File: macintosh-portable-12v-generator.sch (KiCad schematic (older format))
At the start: 14 parts, among them Q3 P2A

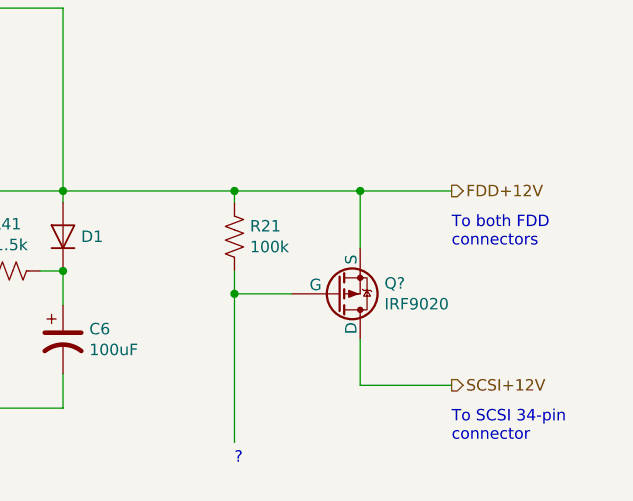
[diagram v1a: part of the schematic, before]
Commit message: Finished V1M, more references on other sheets.
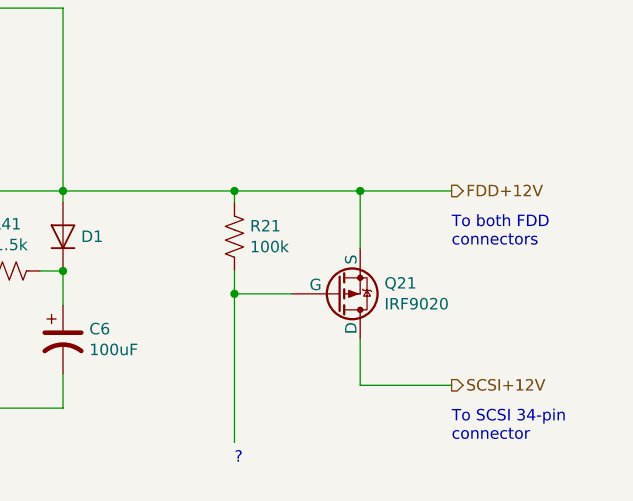
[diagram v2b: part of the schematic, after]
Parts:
- gave numbers to parts that had none: 1
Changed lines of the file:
@@
 Sheet 3 4
 Title "Macintosh Portable 12V Generator Circuit"
-Date "2019-05-22"
-Rev "0.1"
+Date "2019-05-27"
+Rev "0.12"
 Comp "https://oldcrap.org"
-Comment1 ""
+Comment1 "Author: Pawel Pieczul"
 Comment2 ""
 Comment3 ""
@@
 Connection ~ 6400 4350
 $Comp
-L Transistor_FET:IRF9020 Q?
+L Transistor_FET:IRF9020 Q21
 U 1 1 5CFB719D
 P 7600 4450
-F 0 "Q?" H 7806 4404 50  0000 L CNN
+F 0 "Q21" H 7806 4404 50  0000 L CNN
 F 1 "IRF9020" H 7806 4495 50  0000 L CNN
 F 2 "Package_TO_SOT_SMD:TO-252-3_TabPin2" H 7800 4375 50  0001 L CIN

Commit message: Symbol library cleanup
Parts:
- Q21: symbol Transistor_FET:IRF9020 -> macintosh-portable:IRF9020
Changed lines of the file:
@@
 $Descr A4 11693 8268
 encoding utf-8
-Sheet 3 4
+Sheet 3 5
 Title "Macintosh Portable 12V Generator Circuit"
 Date "2019-05-27"
@@
 Connection ~ 6400 4350
 $Comp
-L Transistor_FET:IRF9020 Q21
+L macintosh-portable:IRF9020 Q21
 U 1 1 5CFB719D
 P 7600 4450
